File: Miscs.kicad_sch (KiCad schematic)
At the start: 17 parts, among them J8 MEM2080-00-128-00-A_REVA, Q2 SI7232DN-T1-GE3, U11 XTSD08GLGEAG

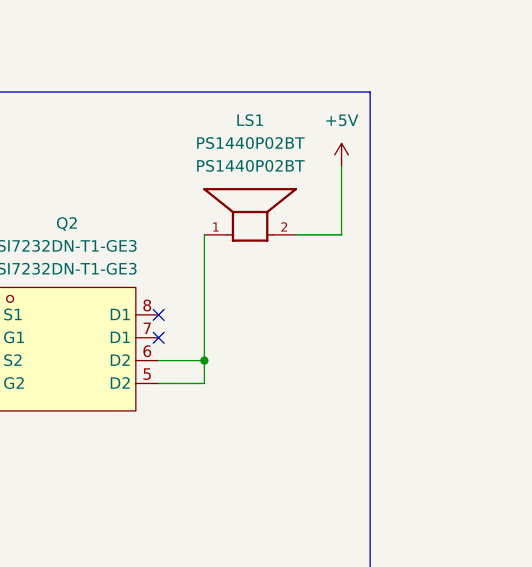
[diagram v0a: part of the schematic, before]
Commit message: adjustments
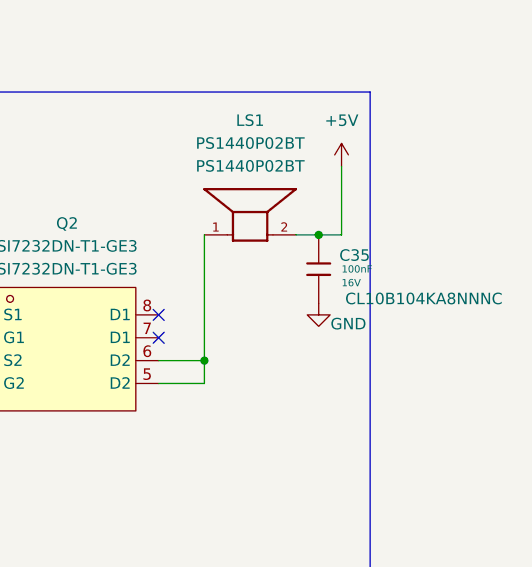
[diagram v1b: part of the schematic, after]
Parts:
- added C35: 100nF, PCM_JLCPCB:C_0603, symbol PCM_JLCPCB-Capacitors:0402,100nF
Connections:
- net +5V: now also C35.1
- net GND: now also C35.2
